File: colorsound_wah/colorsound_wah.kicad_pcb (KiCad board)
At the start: 2 copper layers, 80 x 43 mm, 36 parts, among them Q1 2N2222, SW1 SW_Wuerth_450301014042, U1 40106, U2 VTL5C9

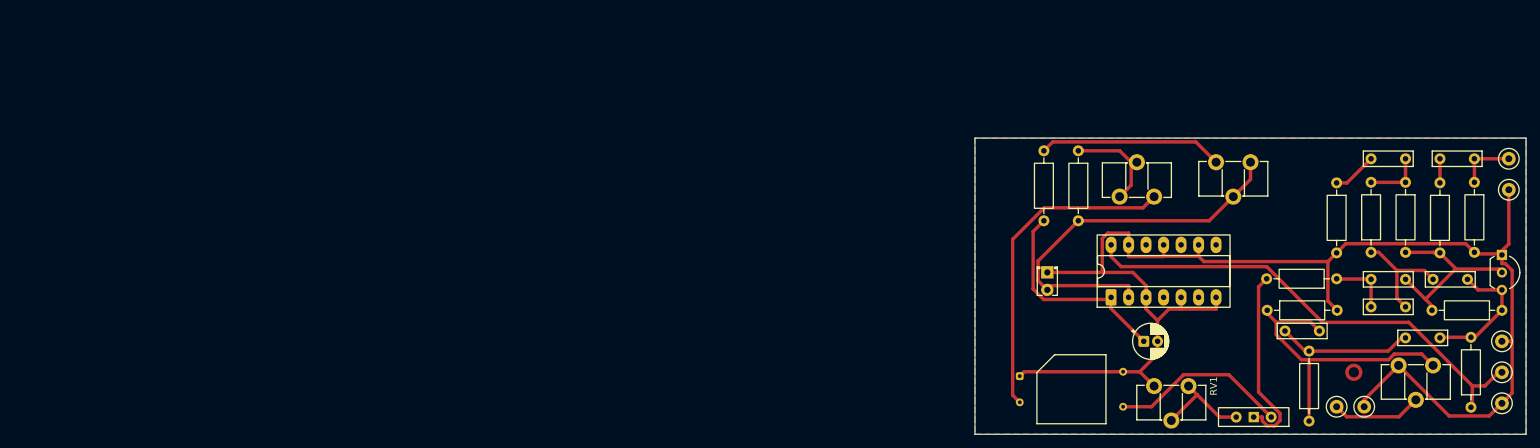
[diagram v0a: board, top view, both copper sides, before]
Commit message: u
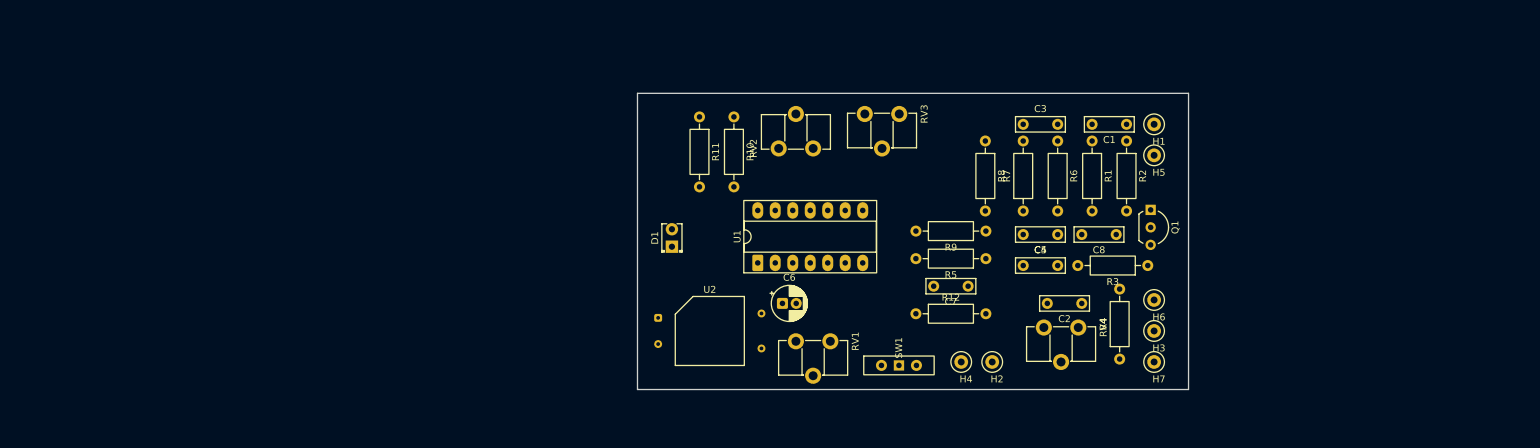
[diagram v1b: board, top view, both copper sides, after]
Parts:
- moved R12 59.2 mm to (166.9, 97.0), turned to 0 degrees
- moved H4 58.9 mm to (173.5, 104.0)
- moved D1 54.6 mm to (131.5, 87.3), turned to 90 degrees
- moved U2 53.2 mm to (129.5, 97.6)
- moved R1 53.0 mm to (192.5, 71.9), turned to -90 degrees
- moved C6 52.7 mm to (147.5, 95.5)
- moved H6 52.7 mm to (201.5, 95.0)
- moved RV1 52.4 mm to (154.5, 101.0)
- moved C2 52.2 mm to (191.0, 95.5)
- moved SW1 52.0 mm to (164.5, 104.5), turned to 0 degrees
- moved R3 51.8 mm to (200.6, 90.0)
- moved RV4 51.8 mm to (190.5, 99.0)
- moved H1 51.7 mm to (201.5, 69.5)
- moved H5 51.7 mm to (201.5, 74.0)
- moved U1 51.5 mm to (144.0, 89.6)
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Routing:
- net GND: track 203.7 -> 0.00 mm
- net VCC: track 70.2 -> 0.00 mm
- net Net-(D1-A): track 56.8 -> 0.00 mm
- net Net-(U2-+): track 47.2 -> 0.00 mm
- net Net-(C7-Pad2): track 45.1 -> 0.00 mm
- net Net-(C6-Pad1): track 30.8 -> 0.00 mm
- net Net-(Q1-B): track 27.6 -> 0.00 mm
- net Net-(SW1-B): track 27.3 -> 0.00 mm
- net Net-(R11-Pad1): track 26.8 -> 0.00 mm
- net Net-(SW1-C): track 26.0 -> 0.00 mm
- net Net-(C2-Pad2): track 19.6 -> 0.00 mm
- net Net-(Q1-C): track 19.4 -> 0.00 mm
- net Net-(C5-Pad2): track 16.4 -> 0.00 mm
- net Net-(R10-Pad1): track 14.9 -> 0.00 mm
- net Net-(SW1-A): track 14.1 -> 0.00 mm
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- removed copper zone on F.Cu, net GND
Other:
- board text removed: "Screw"

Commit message: update
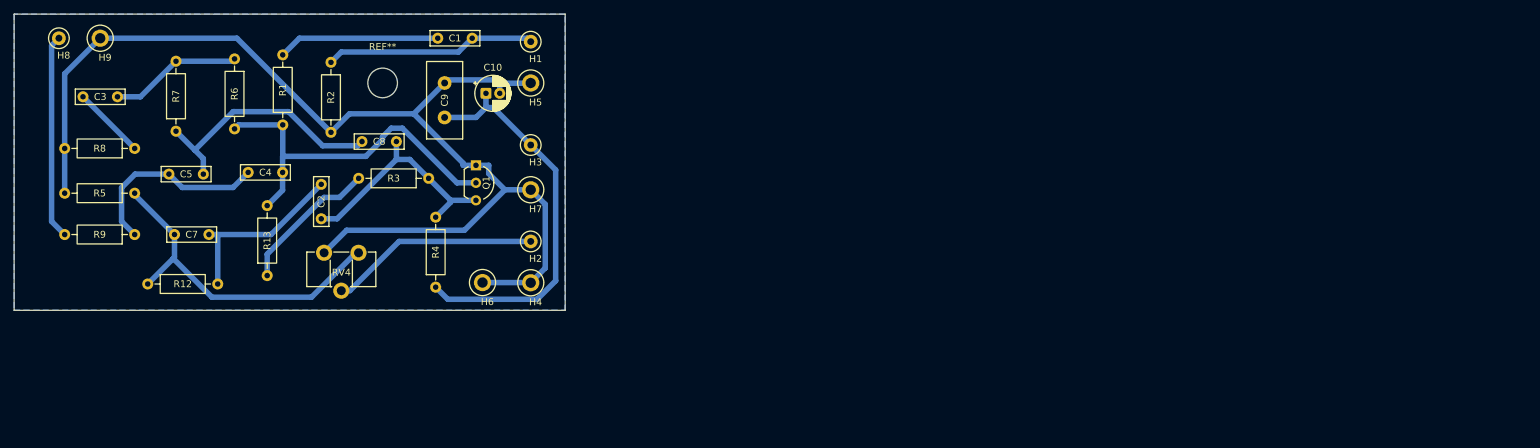
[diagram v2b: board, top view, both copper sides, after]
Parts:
- removed C6: 68u, Capacitor_THT:CP_Radial_D5.0mm_P2.00mm
- removed D1: LED, LED_THT:LED_D2.0mm_W4.0mm_H2.8mm_FlatTop
- removed R10: 2.2K, Resistor_THT:R_Axial_DIN0207_L6.3mm_D2.5mm_P10.16mm_Horizontal
- removed R11: 1K, Resistor_THT:R_Axial_DIN0207_L6.3mm_D2.5mm_P10.16mm_Horizontal
- removed RV1: 100K, Potentiometer_THT:Potentiometer_ACP_CA9-H5_Horizontal
- removed RV2: 10K, Potentiometer_THT:Potentiometer_ACP_CA9-H5_Horizontal
- removed RV3: 25K, Potentiometer_THT:Potentiometer_ACP_CA9-H5_Horizontal
- removed SW1: SW_Wuerth_450301014042, Button_Switch_THT:SW_Slide-03_Wuerth-WS-SLTV_10x2.5x6.4_P2.54mm
- removed U1: 40106, Package_DIP:CERDIP-14_W7.62mm_SideBrazed_LongPads_Socket
- removed U2: VTL5C9, OptoDevice:PerkinElmer_VTL5C
- added C10: 47u, LibraryGabi:CP_Radial_D5.0mm_P2.00mm, F.Cu at (104.5, 65.0)
- added C9: 100n, Capacitor_THT:C_Disc_D11.0mm_W5.0mm_P5.00mm, F.Cu at (98.5, 63.5)
- added H8: POT, TestPoint:TestPoint_Loop_D2.50mm_Drill1.0mm_LowProfile, F.Cu at (42.5, 57.0)
- added H9: GND, LibraryGabi:TestPoint_Loop_D2.50mm_Drill1.85mm, F.Cu at (48.5, 57.0)
- added R13: 1M, LibraryGabi:R_Axial_DIN0207_L6.3mm_D2.5mm_P10.16mm_Horizontal, F.Cu at (72.7, 91.5)
- added REF**: S, MountingHole:MountingHole_4.3mm_M4, F.Cu at (89.5, 63.5)
- C1, C2, C3, C4, C5, C7, C8: footprint Capacitor_THT:C_Rect_L7.0mm_W2.0mm_P5.00mm -> LibraryGabi:C_Rect_L7.0mm_W2.0mm_P5.00mm
- H4, H5, H6, H7: footprint TestPoint:TestPoint_Loop_D2.50mm_Drill1.0mm_LowProfile -> LibraryGabi:TestPoint_Loop_D2.50mm_Drill1.85mm
- R1, R12, R2, R4, R5, R6, R7, R8, R9: footprint Resistor_THT:R_Axial_DIN0207_L6.3mm_D2.5mm_P10.16mm_Horizontal -> LibraryGabi:R_Axial_DIN0207_L6.3mm_D2.5mm_P10.16mm_Horizontal
- R3: value 5.7M -> 2M; footprint Resistor_THT:R_Axial_DIN0207_L6.3mm_D2.5mm_P10.16mm_Horizontal -> LibraryGabi:R_Axial_DIN0207_L6.3mm_D2.5mm_P10.16mm_Horizontal
- RV4: footprint Potentiometer_THT:Potentiometer_ACP_CA9-H5_Horizontal -> LibraryGabi:Potentiometer_ACP_CA9-H5_Horizontal
- moved C3 136.6 mm to (46.0, 65.5)
- moved C5 124.7 mm to (58.5, 76.7)
- moved R5 123.9 mm to (53.5, 79.5)
- moved R9 123.6 mm to (53.5, 85.5)
- moved R7 123.5 mm to (59.5, 70.5)
- moved R8 123.5 mm to (53.5, 73.0), turned to 180 degrees
- moved R6 120.1 mm to (68.0, 60.0)
- moved R1 117.5 mm to (75.0, 69.6), turned to 90 degrees
- moved R2 116.1 mm to (82.0, 60.5)
- moved C4 112.9 mm to (75.0, 76.5)
- moved R12 111.6 mm to (55.4, 92.7)
- moved C2 111.1 mm to (80.6, 83.2), turned to 90 degrees
- moved C7 110.5 mm to (64.3, 85.5)
- moved C8 110.3 mm to (86.5, 72.0), turned to 0 degrees
- moved R3 105.2 mm to (96.2, 77.3)
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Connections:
- R3 pad 2: Net-(Q1-B) -> Net-(R13-Pad1)
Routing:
- net GND: track 0.00 -> 172.3 mm
- net VCC: track 0.00 -> 57.9 mm
- net Net-(Q1-B): track 0.00 -> 53.2 mm
- net Net-(C7-Pad2): track 0.00 -> 49.1 mm
- net Net-(C5-Pad2): track 0.00 -> 36.8 mm
- net Net-(Q1-C): track 0.00 -> 34.4 mm
- net Input guitar: track 0.00 -> 30.7 mm
- net Output: track 0.00 -> 30.5 mm
- net Net-(H8-Pad1): track 0.00 -> 29.7 mm
- net Net-(C4-Pad2): track 0.00 -> 28.5 mm
- net Net-(C2-Pad2): track 0.00 -> 26.5 mm
- net Net-(C1-Pad2): track 0.00 -> 23.5 mm
- net Net-(R13-Pad1): track 0.00 -> 20.9 mm
- net Net-(C3-Pad2): track 0.00 -> 19.3 mm
- net Net-(C3-Pad1): track 0.00 -> 10.6 mm
- added copper zone on B.Cu, net GND
